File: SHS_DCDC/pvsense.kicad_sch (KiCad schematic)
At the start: 9 parts, among them U3 LMV324AIDR

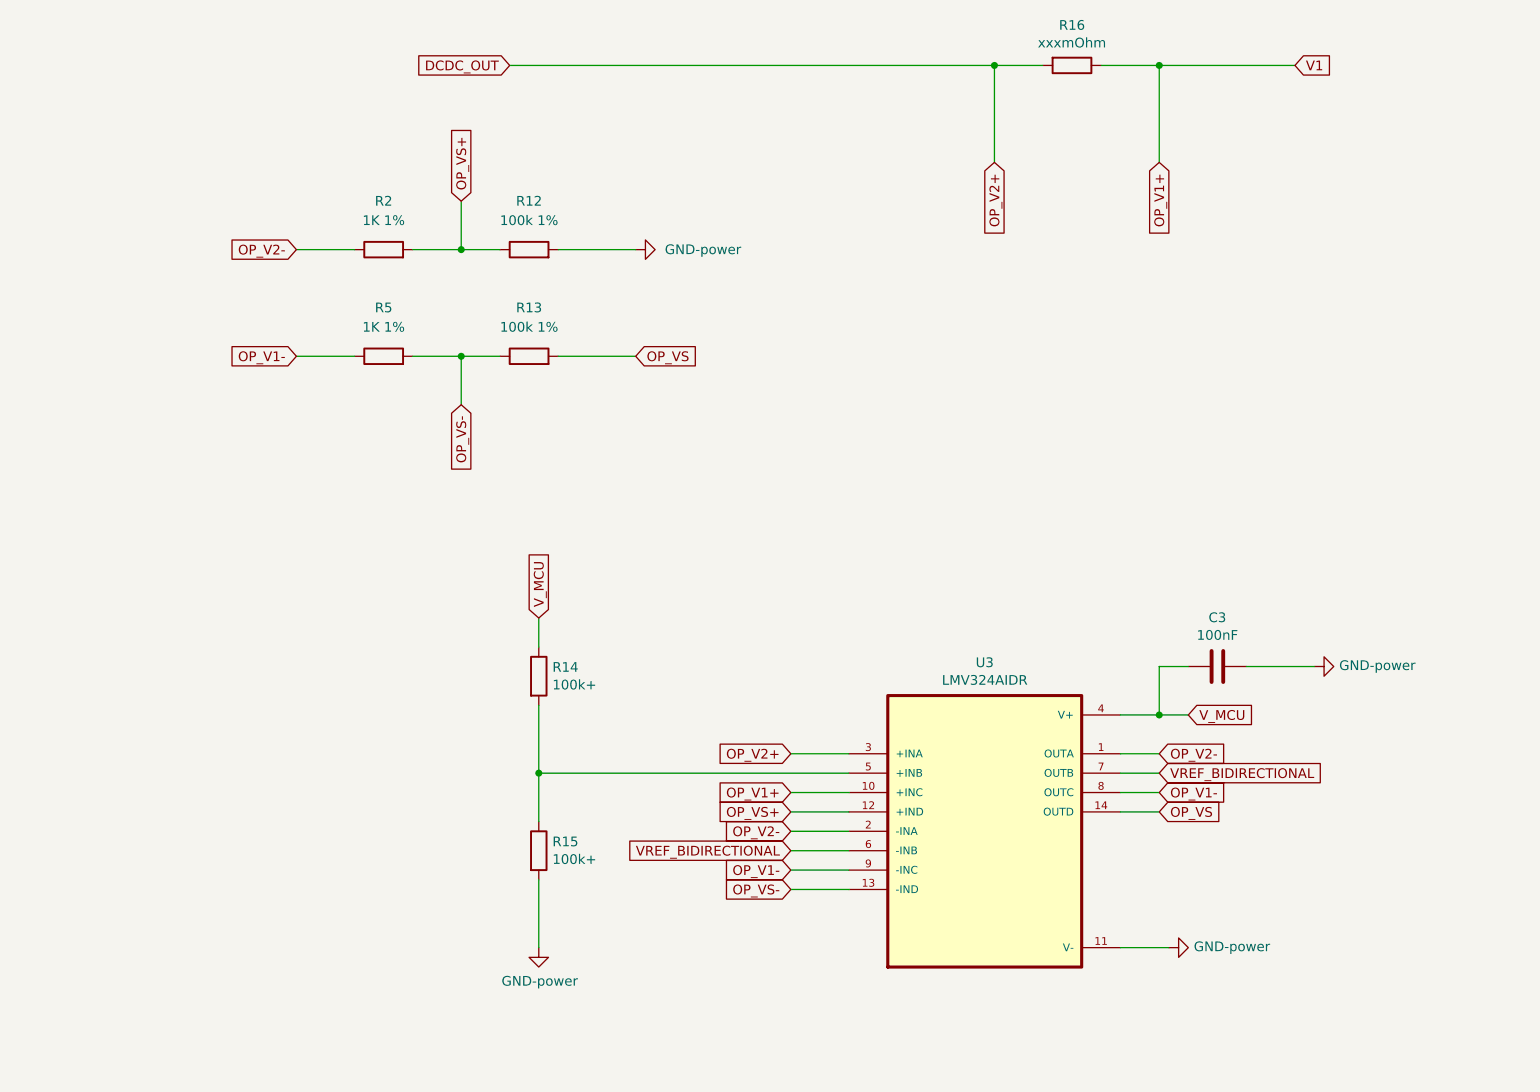
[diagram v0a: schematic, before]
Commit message: Commit_190223
Normal commit
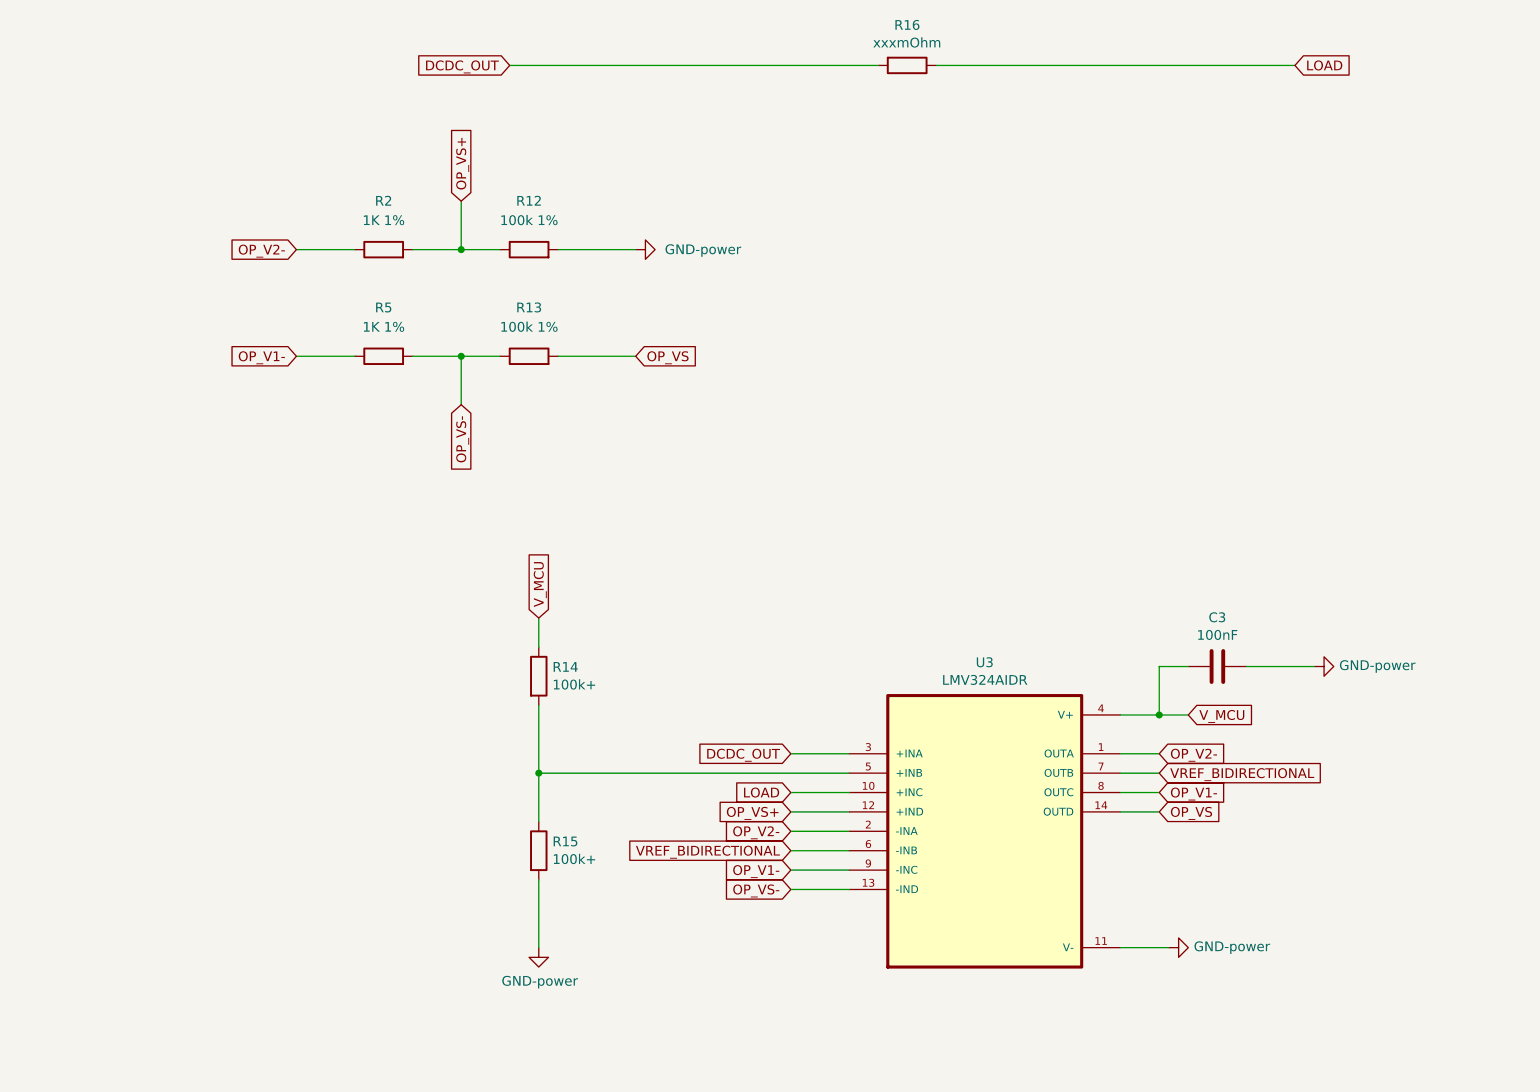
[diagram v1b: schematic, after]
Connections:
- net OP_V1+ renamed LOAD
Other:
- moved on the sheet: R16
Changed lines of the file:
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@@
   (junction (at 180.34 118.11) (diameter 0) (color 0 0 0 0)
   )
-  (junction (at 180.34 33.02) (diameter 0) (color 0 0 0 0)
-  )
-  (junction (at 158.75 33.02) (diameter 0) (color 0 0 0 0)
-  )
   (wire (pts (xy 99.06 125.73) (xy 99.06 116.84))
     (stroke (width 0) (type default) (color 0 0 0 0))
@@
     (stroke (width 0) (type default) (color 0 0 0 0))
   )
-  (wire (pts (xy 180.34 33.02) (xy 198.12 33.02))
-    (stroke (width 0) (type default) (color 0 0 0 0))
-  )
   (wire (pts (xy 99.06 139.7) (xy 99.06 148.59))
     (stroke (width 0) (type default) (color 0 0 0 0))
@@
     (stroke (width 0) (type default) (color 0 0 0 0))
   )
-  (wire (pts (xy 180.34 33.02) (xy 180.34 45.72))
-    (stroke (width 0) (type default) (color 0 0 0 0))
-  )
-  (wire (pts (xy 158.75 33.02) (xy 158.75 45.72))
-    (stroke (width 0) (type default) (color 0 0 0 0))
-  )
   (wire (pts (xy 180.34 118.11) (xy 184.15 118.11))
     (stroke (width 0) (type default) (color 0 0 0 0))
@@
     (stroke (width 0) (type default) (color 0 0 0 0))
   )
-  (wire (pts (xy 165.1 33.02) (xy 158.75 33.02))
-    (stroke (width 0) (type default) (color 0 0 0 0))
-  )
   (wire (pts (xy 88.9 71.12) (xy 88.9 77.47))
     (stroke (width 0) (type default) (color 0 0 0 0))
@@
     (stroke (width 0) (type default) (color 0 0 0 0))
   )
-  (wire (pts (xy 158.75 33.02) (xy 95.25 33.02))
+  (wire (pts (xy 95.25 33.02) (xy 143.51 33.02))
     (stroke (width 0) (type default) (color 0 0 0 0))
   )
@@
     (stroke (width 0) (type default) (color 0 0 0 0))
   )
-  (wire (pts (xy 180.34 33.02) (xy 172.72 33.02))
+  (wire (pts (xy 151.13 33.02) (xy 198.12 33.02))
     (stroke (width 0) (type default) (color 0 0 0 0))
   )
@@
     )
   )
-  (global_label "OP_V2+" (shape input) (at 132.08 123.19 180) (fields_autoplaced)
-    (effects (font (size 1.27 1.27)) (justify right))
-    (property "Intersheet References" "${INTERSHEET_REFS}" (id 0) (at 122.3172 123.1106 0)
+  (global_label "DCDC_OUT" (shape input) (at 132.08 123.19 180) (fields_autoplaced)
+    (effects (font (size 1.27 1.27)) (justify right))
+    (property "Intersheet References" "${INTERSHEET_REFS}" (id 0) (at 120.0796 123.1106 0)
       (effects (font (size 1.27 1.27)) (justify right) hide)
     )
@@
     )
   )
-  (global_label "OP_V1+" (shape input) (at 180.34 45.72 270) (fields_autoplaced)
-    (effects (font (size 1.27 1.27)) (justify right))
-    (property "Intersheet References" "${INTERSHEET_REFS}" (id 0) (at 180.2606 55.4828 90)
-      (effects (font (size 1.27 1.27)) (justify right) hide)
-    )
-  )
   (global_label "OP_V2-" (shape input) (at 180.34 123.19 0) (fields_autoplaced)
     (effects (font (size 1.27 1.27)) (justify left))
@@
     )
   )
-  (global_label "V1" (shape input) (at 198.12 33.02 0) (fields_autoplaced)
-    (effects (font (size 1.27 1.27)) (justify left))
-    (property "Intersheet References" "${INTERSHEET_REFS}" (id 0) (at 202.7423 32.9406 0)
+  (global_label "LOAD" (shape input) (at 198.12 33.02 0) (fields_autoplaced)
+    (effects (font (size 1.27 1.27)) (justify left))
+    (property "Intersheet References" "${INTERSHEET_REFS}" (id 0) (at 205.1613 32.9406 0)
       (effects (font (size 1.27 1.27)) (justify left) hide)
     )
@@
     )
   )
-  (global_label "OP_V1+" (shape input) (at 132.08 128.27 180) (fields_autoplaced)
-    (effects (font (size 1.27 1.27)) (justify right))
-    (property "Intersheet References" "${INTERSHEET_REFS}" (id 0) (at 122.3172 128.1906 0)
+  (global_label "LOAD" (shape input) (at 132.08 128.27 180) (fields_autoplaced)
+    (effects (font (size 1.27 1.27)) (justify right))
+    (property "Intersheet References" "${INTERSHEET_REFS}" (id 0) (at 125.0387 128.1906 0)
       (effects (font (size 1.27 1.27)) (justify right) hide)
     )
@@
     (effects (font (size 1.27 1.27)) (justify right))
     (property "Intersheet References" "${INTERSHEET_REFS}" (id 0) (at 57.5472 71.0406 0)
-      (effects (font (size 1.27 1.27)) (justify right) hide)
-    )
-  )
-  (global_label "OP_V2+" (shape input) (at 158.75 45.72 270) (fields_autoplaced)
-    (effects (font (size 1.27 1.27)) (justify right))
-    (property "Intersheet References" "${INTERSHEET_REFS}" (id 0) (at 158.6706 55.4828 90)
       (effects (font (size 1.27 1.27)) (justify right) hide)
     )
@@
     (pin "1")
   )
-  (symbol (lib_id "SHS_DCDC:R-Device") (at 168.91 33.02 270) (unit 1)
+  (symbol (lib_id "SHS_DCDC:R-Device") (at 147.32 33.02 270) (unit 1)
     (in_bom yes) (on_board yes)
-    (property "Reference" "R16" (id 0) (at 168.91 27.7622 90))
-    (property "Value" "xxxmOhm" (id 1) (at 168.91 30.0736 90))
-    (property "Footprint" "Resistor_SMD:R_1206_3216Metric" (id 2) (at 168.91 31.242 90)
-      (effects (font (size 1.27 1.27)) hide)
-    )
-    (property "Datasheet" "~" (id 3) (at 168.91 33.02 0)
-      (effects (font (size 1.27 1.27)) hide)
-    )
+    (property "Reference" "R16" (id 0) (at 147.32 27.7622 90))
+    (property "Value" "xxxmOhm" (id 1) (at 147.32 30.0736 90))
+    (property "Footprint" "Resistor_SMD:R_1206_3216Metric" (id 2) (at 147.32 31.242 90)
+      (effects (font (size 1.27 1.27)) hide)
+    )
+    (property "Datasheet" "~" (id 3) (at 147.32 33.02 0)
+      (effects (font (size 1.27 1.27)) hide)
+    )

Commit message: Commit_190223_2
Commit before checking one older schematic
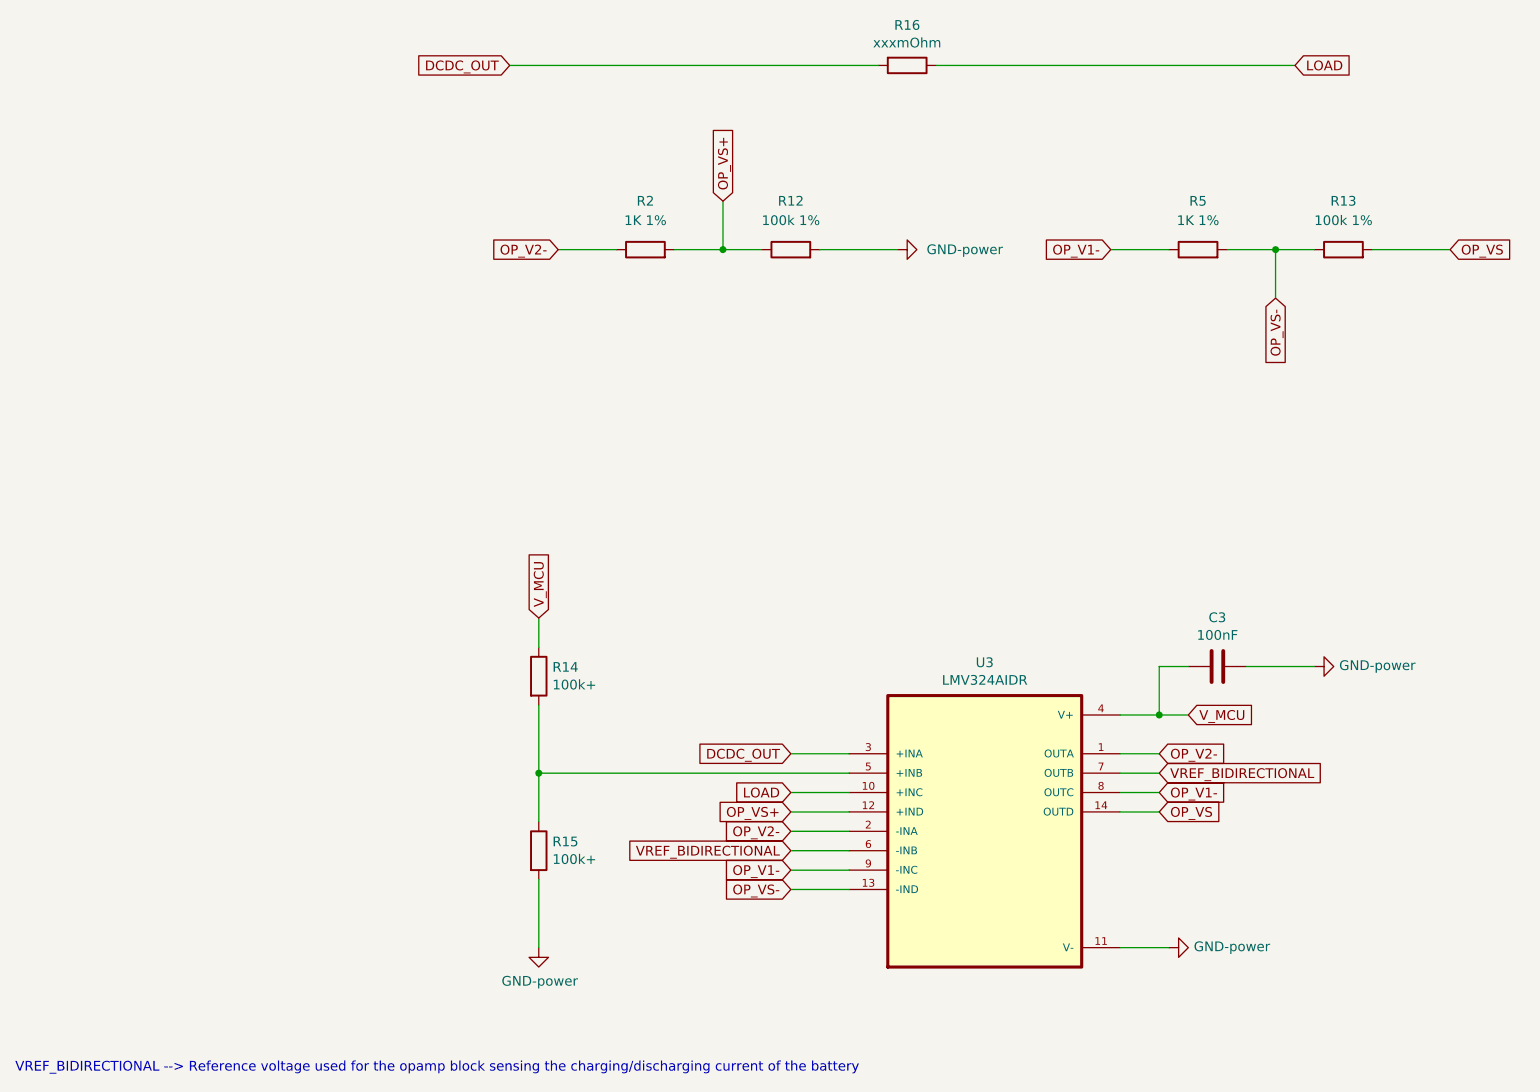
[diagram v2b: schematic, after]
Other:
- note added: "VREF_BIDIRECTIONAL --> Reference voltage used for the opamp block sensing the charging/discharging current of the battery"
- moved on the sheet: R12, R13, R2, R5
